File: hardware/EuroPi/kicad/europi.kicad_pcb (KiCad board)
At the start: 2 copper layers, 85.7 x 110 mm, 92 parts, among them IC1 TL074, IC2 TL074, IC3 MCP6002, J1 Thonkiconn_Mono_Jack, J2 Thonkiconn_Mono_Jack, J3 Thonkiconn_Mono_Jack, J4 Thonkiconn_Mono_Jack, J5 Thonkiconn_Mono_Jack, J6 Thonkiconn_Mono_Jack, J7 Thonkiconn_Mono_Jack, J8 Thonkiconn_Mono_Jack, Q1 2N2222, SW1 SW_Push, SW2 SW_Push

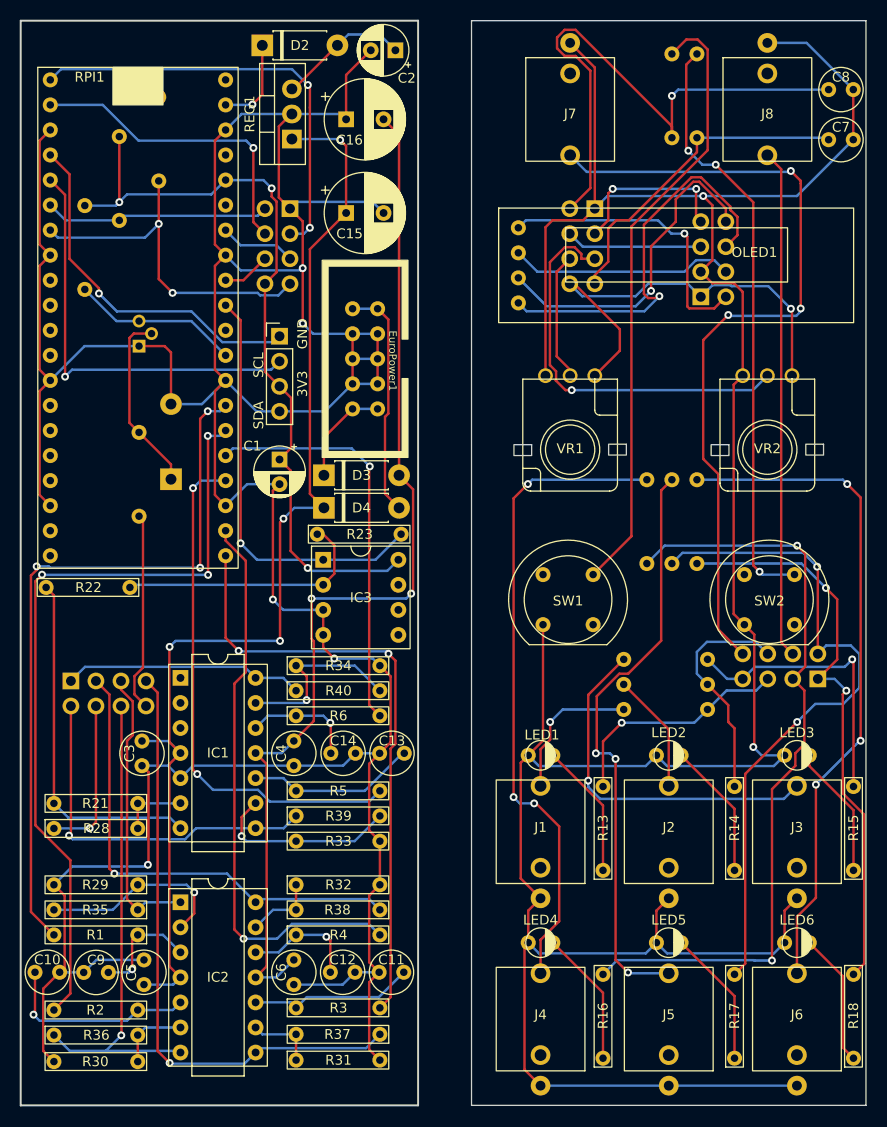
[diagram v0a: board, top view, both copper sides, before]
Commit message: kicad save
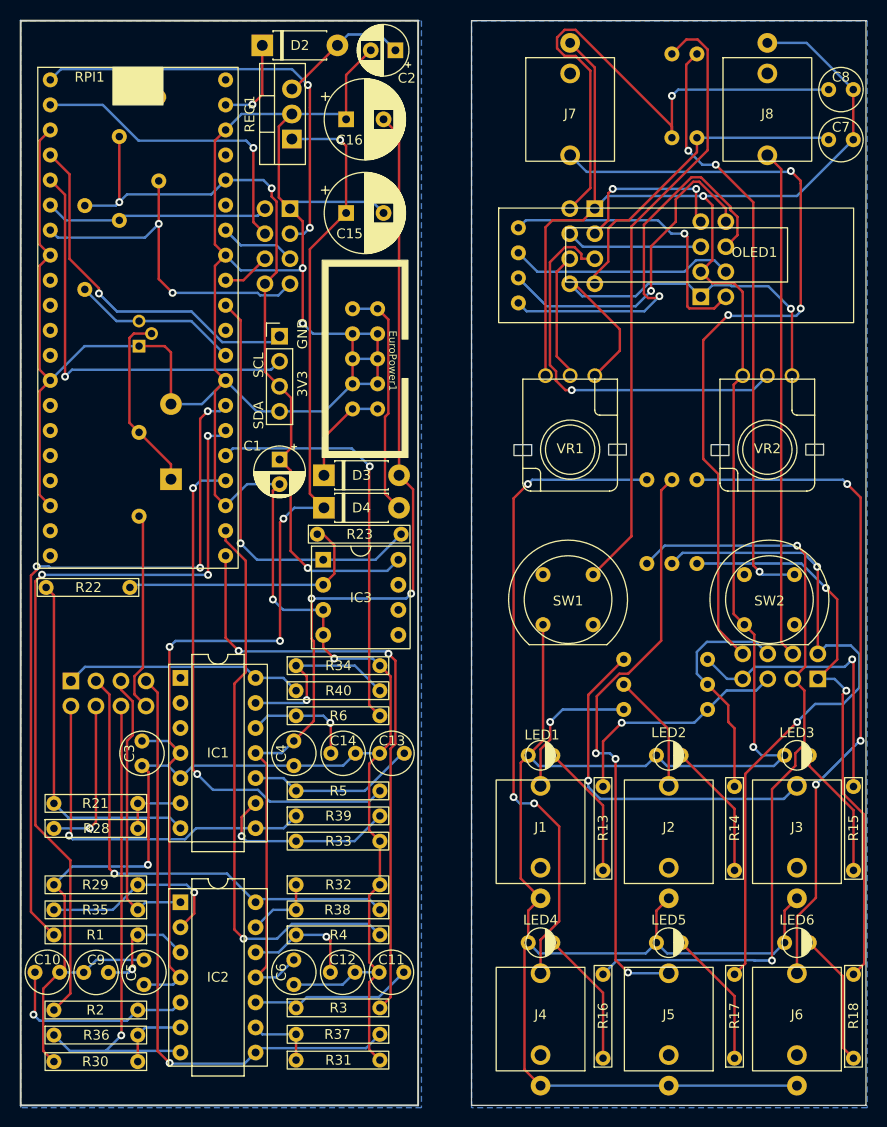
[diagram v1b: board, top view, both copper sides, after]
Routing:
- added copper zone on B.Cu, net /EARTH J
- added copper zone on B.Cu, net Earth
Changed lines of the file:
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@@
   (segment (start 10 36) (end 10.3 35.7) (width 0.25) (layer "F.Cu") (net 107))
   (segment (start 8.636 34.036) (end 8.636 25.464) (width 0.25) (layer "F.Cu") (net 107))
+  (zone (net 1) (net_name "Earth") (layer "B.Cu") (hatch edge 0.5)
+    (priority 1)
+    (connect_pads (clearance 0.508))
+    (min_thickness 0.25) (filled_areas_thickness no)
+    (fill yes (thermal_gap 0.5) (thermal_bridge_width 0.5))
+    (polygon
+      (pts
+        (xy -45.72 0)
+        (xy -5.08 0)
+        (xy -5.08 110.236)
+        (xy -45.72 110.236)
+      )
+    )
+  )
+  (zone (net 105) (net_name "/EARTH J") (layer "B.Cu") (hatch edge 0.5)
+    (connect_pads (clearance 0.508))
+    (min_thickness 0.25) (filled_areas_thickness no)
+    (fill yes (thermal_gap 0.5) (thermal_bridge_width 0.5))
+    (polygon
+      (pts
+        (xy 0 0)
+        (xy 40.132 0)
+        (xy 40.132 110.236)
+        (xy 0 110.236)
+      )
+    )
+  )
 )
